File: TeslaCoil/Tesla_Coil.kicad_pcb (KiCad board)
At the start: 4 copper layers, 200 x 97.5 mm, 37 parts, among them J1 SOLAR_INPUT, J2 SOLAR_OUTPUT, J3 Left, J4 Right, J5 5V, J6 BATTERY_INPUT, J7 BATTERY_OUTPUT, Q1 Q_NPN_BCE, Q4 IRFIZ44N

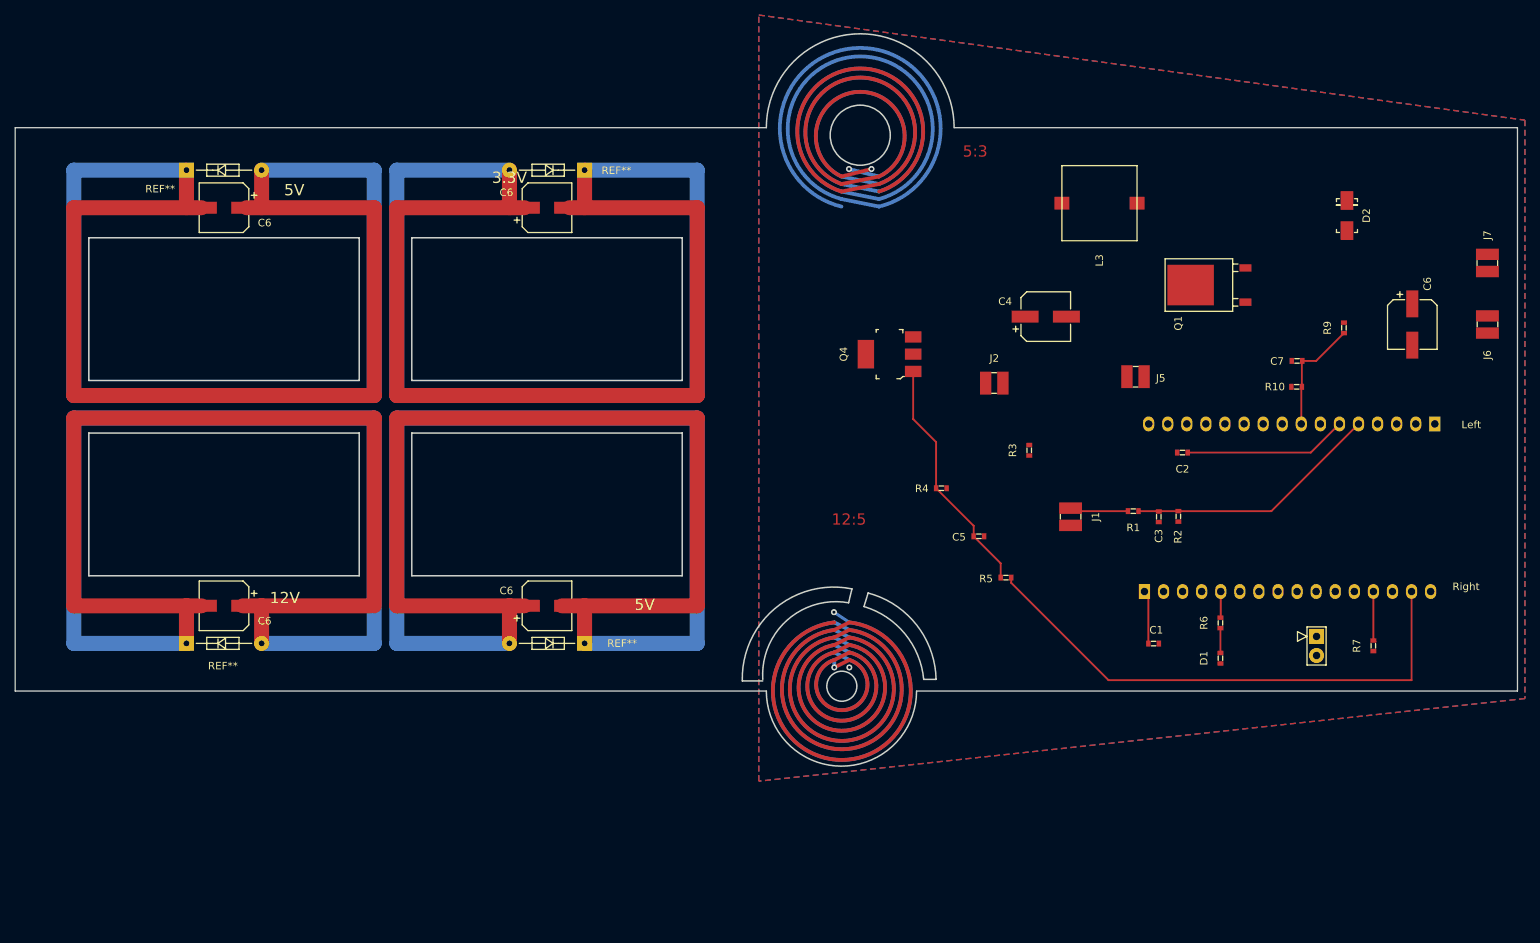
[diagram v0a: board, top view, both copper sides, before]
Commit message: save
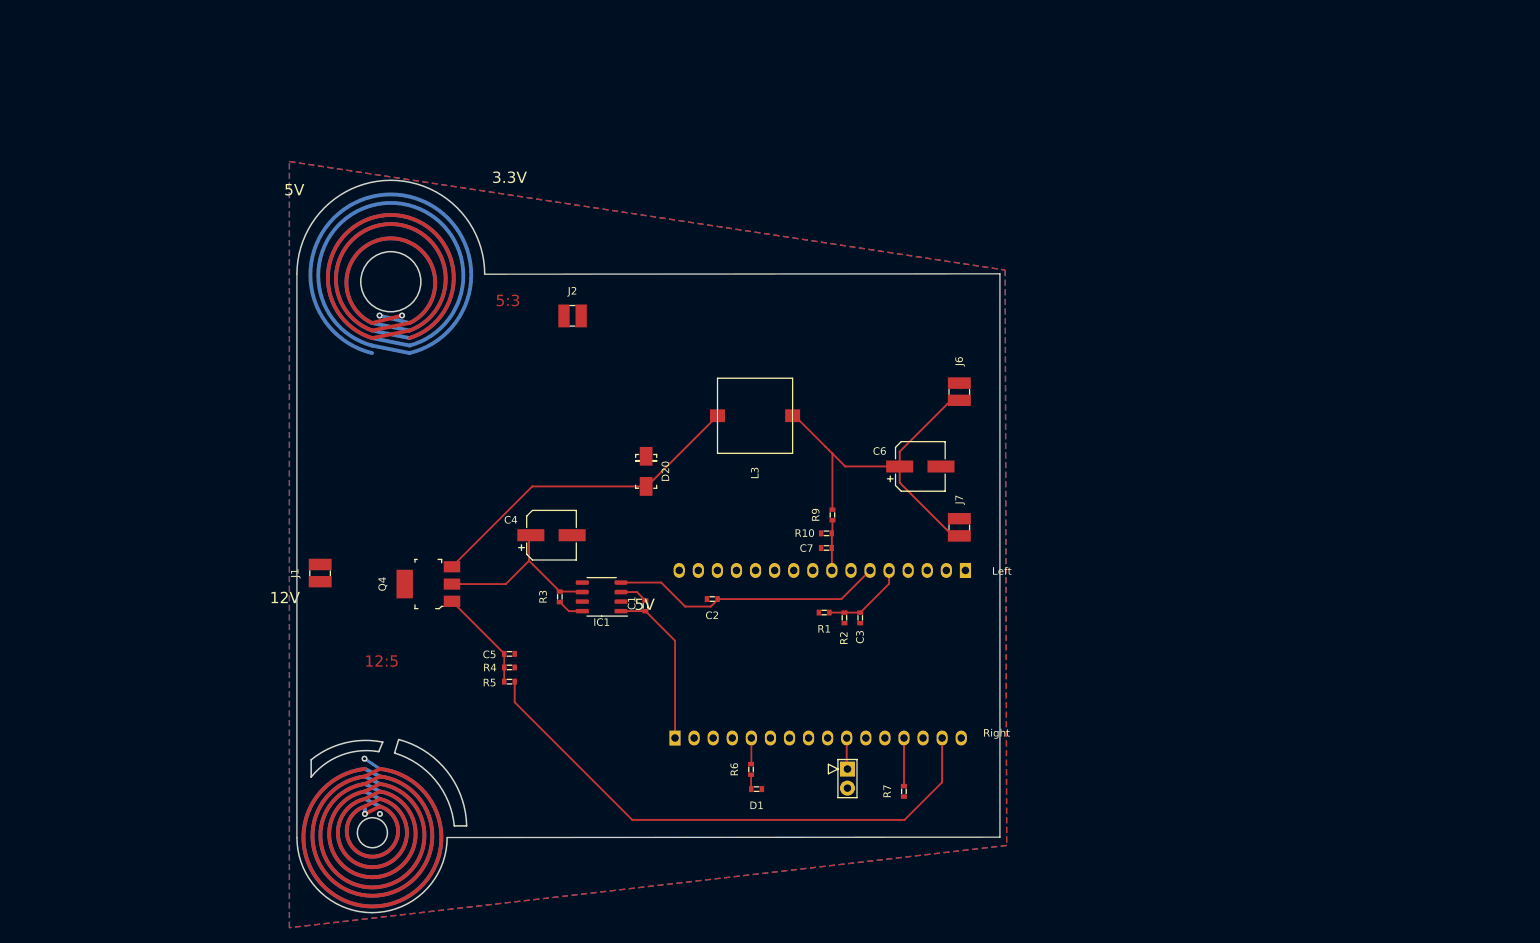
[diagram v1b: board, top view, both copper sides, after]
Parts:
- removed the C6 at (139.0, 89.0)
- removed the C6 at (182.0, 142.0)
- removed the C6 at (139.0, 142.0)
- removed the C6 at (182.0, 89.0)
- removed J5: 5V, digikey-footprints:1210
- removed Q1: Q_NPN_BCE, ESP32-footprints-Lib:Dpak
- removed REF** (x4): Diode_DO-35_P10mm, digikey-footprints:Diode_DO-35_P10mm
- added IC1: MAX4173H, Package_SO:SO-8_3.9x4.9mm_P1.27mm, F.Cu at (189.3, 140.8)
- moved J1 100.2 mm to (151.8, 137.6), turned to 90 degrees
- moved D20 99.3 mm to (195.2, 124.1)
- moved J7 78.6 mm to (236.9, 131.5)
- moved R9 72.5 mm to (220.0, 129.9)
- moved C4 71.9 mm to (182.6, 132.6)
- moved J6 70.9 mm to (236.9, 113.5), turned to 90 degrees
- moved Q4 68.6 mm to (166.2, 139.1)
- moved C6 68.2 mm to (231.7, 123.4), turned to 180 degrees
- moved C1 67.8 mm to (195.1, 142.0), turned to 90 degrees
- moved R5 67.5 mm to (177.0, 152.1)
- moved C7 67.4 mm to (219.2, 134.3)
- moved C2 65.6 mm to (204.0, 141.1)
- moved R10 65.6 mm to (219.2, 132.3)
- moved R6 65.5 mm to (209.2, 163.8)
- moved J4 65.5 mm to (219.4, 158.3)
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- renumbered D2 to D20
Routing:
- net Bat+: track 0.00 -> 50.0 mm
- net Net-(D20-K): track 0.00 -> 43.7 mm
- net +12V: track 0.00 -> 23.4 mm
- net U_Sol: track 34.1 -> 11.3 mm
- net Net-(Q4-G): track 32.3 -> 13.7 mm
- net +3V3: track 7.15 -> 22.5 mm
- net I_Sol: track 21.8 -> 36.5 mm
- net U_Bat: track 15.5 -> 6.83 mm
- net Net-(IC1-RS+): track 8.51 -> 3.50 mm
- net Net-(J4-Pin_10): track 0.00 -> 4.17 mm
- net GND: track 0.00 -> 3.72 mm
- net PWM: track 71.2 -> 74.1 mm
- net Net-(D1-A): track 3.30 -> 1.93 mm
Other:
- board size 200 x 97.5 mm -> 93.6 x 97.5 mm
